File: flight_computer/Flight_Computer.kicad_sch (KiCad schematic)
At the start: 112 parts

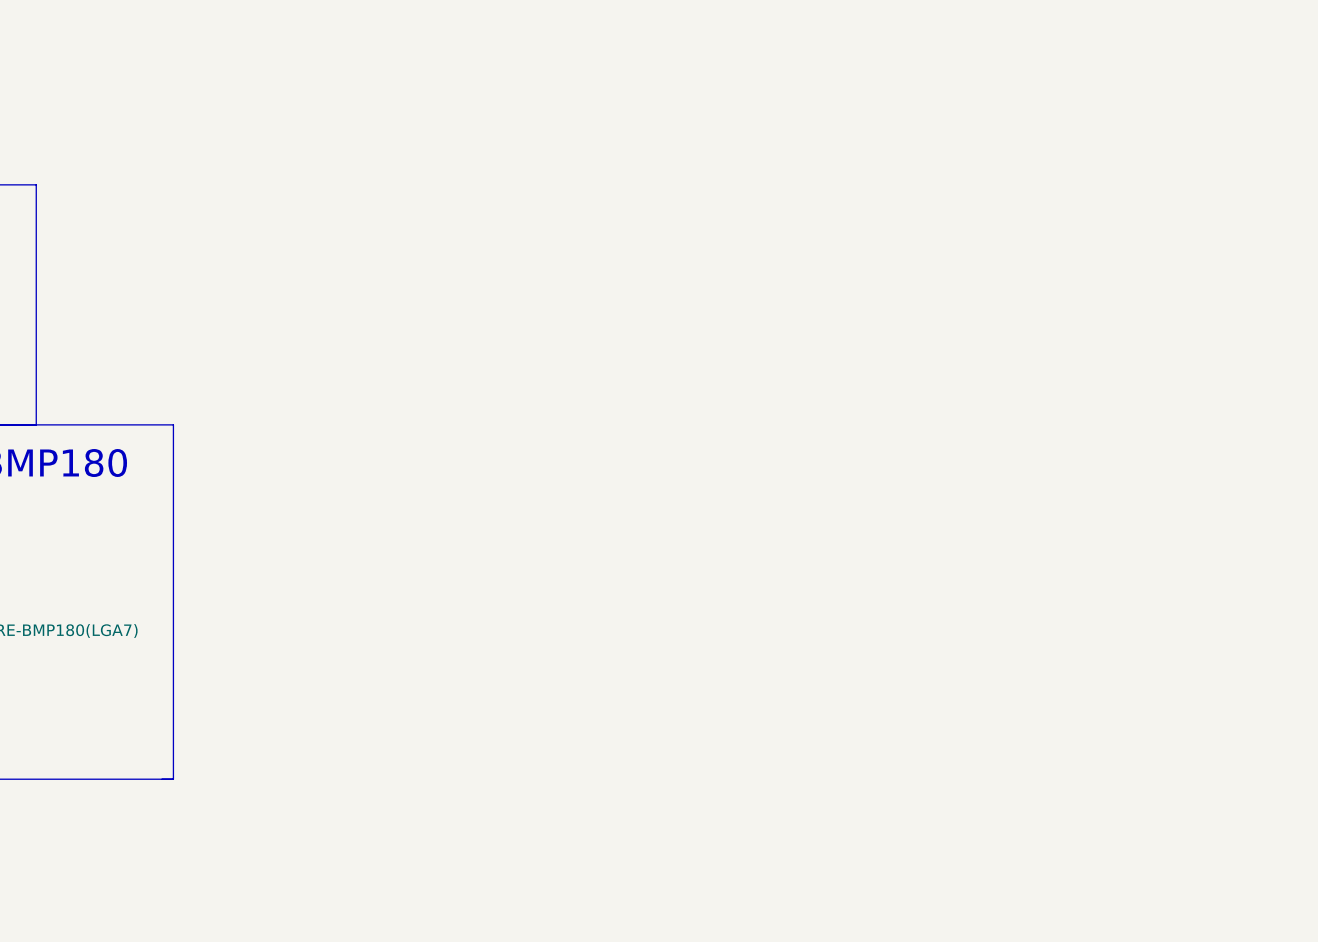
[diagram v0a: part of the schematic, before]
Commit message: bakerw
ignitor
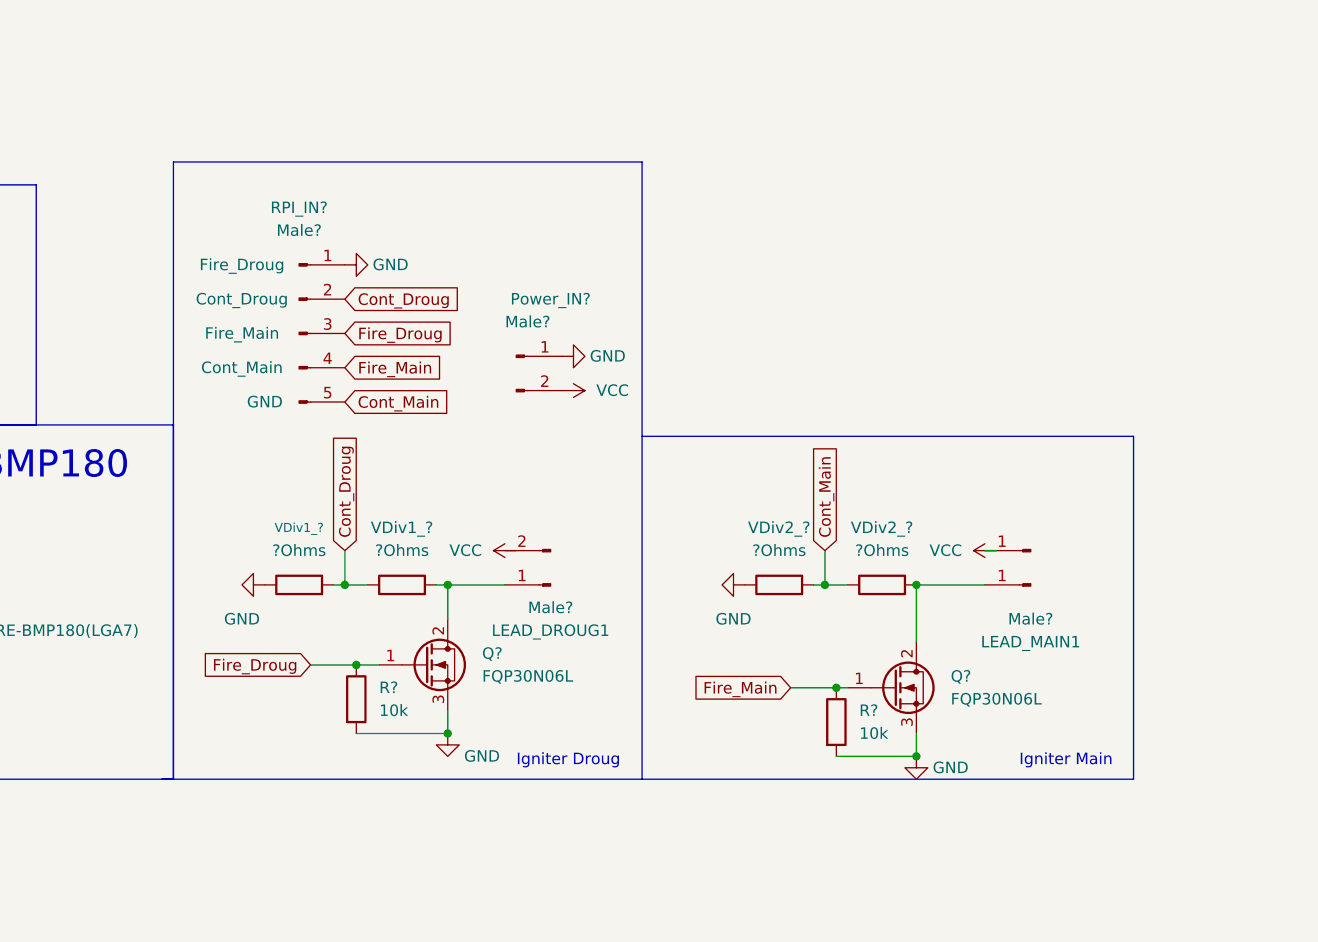
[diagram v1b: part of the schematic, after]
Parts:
- added Male?: LEAD_MAIN1, symbol Connector:Conn_01x01_Male
- added Male?: LEAD_DROUG1, symbol Connector:Conn_01x01_Male
- added Male? (x2): Fire_Droug, symbol Connector:Conn_01x01_Male
- added Male? (x2): Male, symbol Connector:Conn_01x01_Male
- added Power_IN?, RPI_IN?: Cont_Droug, symbol Connector:Conn_01x01_Male
- added Q? (x2): FQP30N06L, Package_TO_SOT_THT:TO-220-3_Vertical, symbol Transistor_FET:FQP27P06
- added R? (x2): 10k, symbol Device:R
- added RPI_IN?: Fire_Main, symbol Connector:Conn_01x01_Male
- added RPI_IN?: Cont_Main, symbol Connector:Conn_01x01_Male
- added RPI_IN?: GND, symbol Connector:Conn_01x01_Male
- added VDiv1_? (x2), VDiv2_? (x2): ?Ohms, symbol Device:R
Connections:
- net GND: now also Male?.1 (Pin_1), Male?.1 (Pin_1), Q?.3 (S), Q?.3 (S), R?.2, R?.2, VDiv1_?.1, VDiv2_?.1
- new net: Male?.1 (Pin_1), Q?.2 (D), VDiv2_?.2
- new net: Male?.1 (Pin_1), Q?.2 (D), VDiv1_?.2
- new net Cont_Droug: RPI_IN?.2 (Pin_1), VDiv1_?.1, VDiv1_?.2
- new net Cont_Main: RPI_IN?.5 (Pin_1), VDiv2_?.1, VDiv2_?.2
- new net Fire_Droug: Q?.1 (G), R?.1, RPI_IN?.3 (Pin_1)
- new net Fire_Main: Q?.1 (G), R?.1, RPI_IN?.4 (Pin_1)
- new net VCC: Male?.1 (Pin_1), Power_IN?.2 (Pin_1)
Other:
- note added: "Igniter Droug"
- note added: "Igniter Main"
